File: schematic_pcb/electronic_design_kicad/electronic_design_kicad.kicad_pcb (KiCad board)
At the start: 2 copper layers, 34.2 x 13.6 mm, 20 parts, among them IC1 ATTINY85-S, P1 USB_A, P2 CONN_6

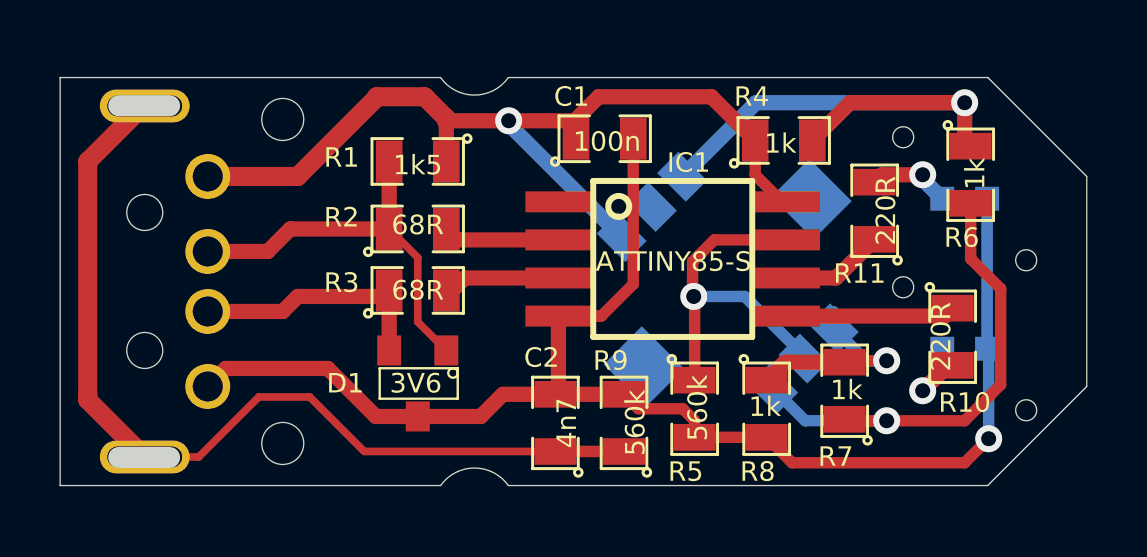
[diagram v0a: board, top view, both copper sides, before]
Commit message: hardware revision 3.0
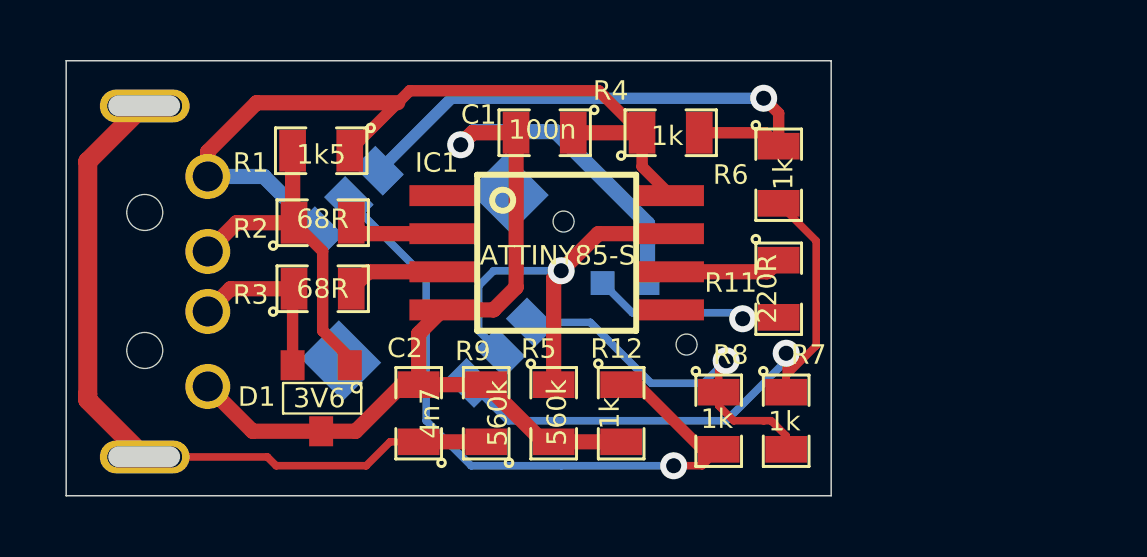
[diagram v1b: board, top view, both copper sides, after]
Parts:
- removed D2: LED GREEN, projectLib:LED_0603_PIPE
- removed R10: 220R, projectLib:SMD-0805
- added R12: 1k, projectLib:SMD-0805, F.Cu at (156.8, 186.8)
- P2: footprint SKRHAAE010 -> projectLib:SKRHAAE010
- moved D3 11.7 mm to (156.9, 182.4)
- moved P2 10.1 mm to (150.2, 182.2)
- moved area0x33 9.73 mm to (159.5, 178.2)
- moved R6 6.40 mm to (162.0, 178.8)
- moved R5 4.70 mm to (154.5, 186.8)
- moved R9 4.61 mm to (152.2, 186.8)
- moved C2 4.57 mm to (150.0, 186.8)
- moved R11 4.12 mm to (162.0, 182.6), turned to 270 degrees
- moved IC1 3.87 mm to (154.6, 181.4)
- moved R4 3.78 mm to (158.4, 177.4)
- moved D1 3.26 mm to (146.8, 186.2)
- moved R1 3.24 mm to (146.8, 178.0)
- moved R2 3.18 mm to (146.8, 180.4)
- moved R3 3.17 mm to (146.8, 182.6)
- moved R7 2.19 mm to (162.2, 187.0), turned to 270 degrees
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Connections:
- IC1 pad 5: /G -> (no net)
- P2 pad 2: (no net) -> /CENTER
- R8 pad 2: DGND -> /CENTER
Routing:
- net /CENTER: track 0.00 -> 23.2 mm, vias 0 -> 1
- net DGND: track 47.3 -> 38.2 mm
- net /G: track 5.65 -> 0.00 mm
- net /LEFT: track 7.04 -> 12.4 mm
- net Net-(C2-Pad1): track 30.9 -> 25.6 mm
- net +5V: track 32.5 -> 28.7 mm, vias 1 -> 0
- net Net-(D3-Pad2): track 2.77 -> 6.38 mm
- net Net-(D2-Pad2): track 3.02 -> 0.00 mm, vias 1 -> 0
- net D+: track 8.25 -> 5.34 mm
- net /DOWN: track 17.8 -> 20.7 mm
- net D-: track 13.4 -> 11.2 mm
- net /ADC: track 12.1 -> 13.6 mm
- net /UP: track 17.6 -> 18.5 mm
- net Net-(IC1-Pad3): track 3.99 -> 3.27 mm
- net Net-(IC1-Pad2): track 3.89 -> 3.21 mm
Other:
- board size 34.2 x 13.6 mm -> 25.5 x 14.5 mm
